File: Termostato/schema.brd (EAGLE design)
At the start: 100 x 80 mm, 11 parts, among them K1 RELAY-SPDT-JZC-11F

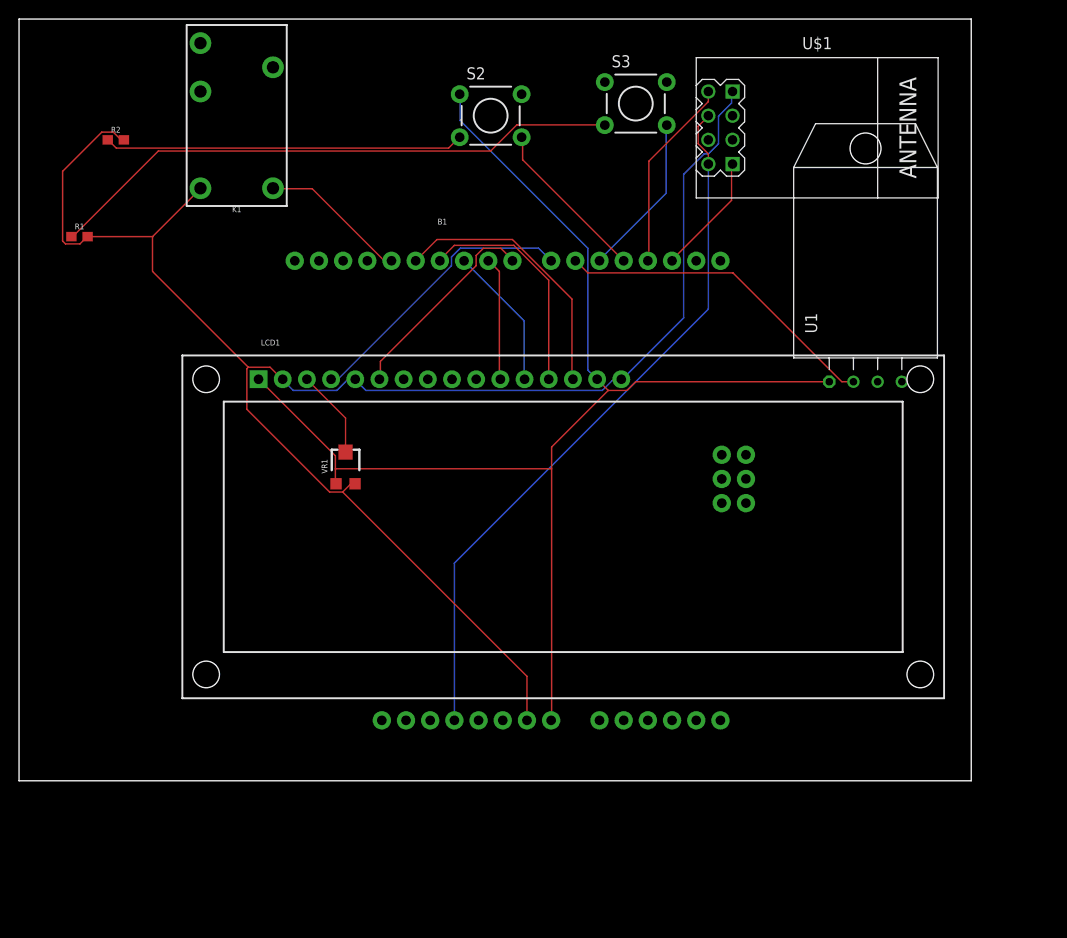
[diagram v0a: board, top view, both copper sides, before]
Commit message: Arduino shield
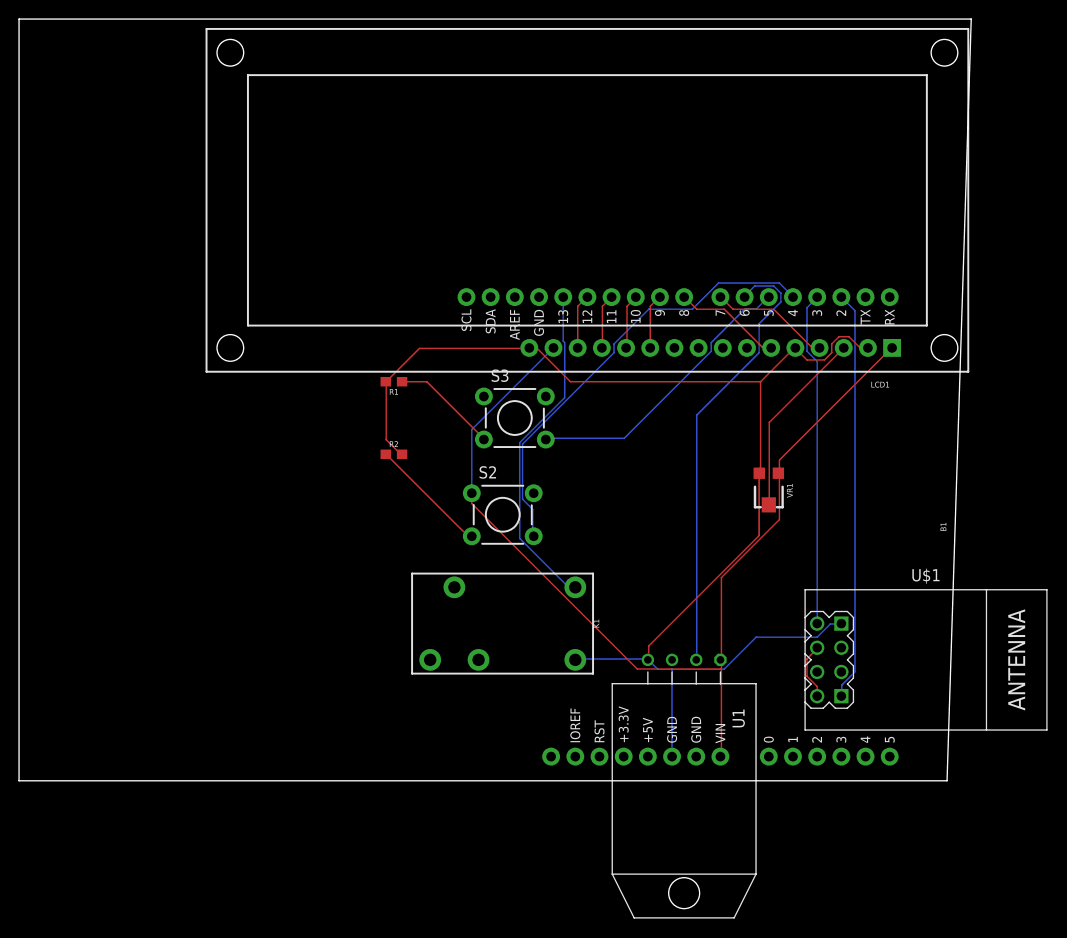
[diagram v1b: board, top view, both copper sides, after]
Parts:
- B1: value ARDUINO_UNO_R3NO_HOLES -> ARDUINO_UNO_R3_SHIELDBASIC; device SparkFun-Boards:ARDUINO_R3_NO_HOLES -> SparkFun-Boards:UNO_R3_SHIELD
- moved K1 60.8 mm to (49.5, 16.5), turned to 90 degrees
- moved U$1 57.0 mm to (95.2, 12.7)
- moved VR1 44.5 mm to (78.7, 30.5), turned to 180 degrees
- moved R2 44.1 mm to (39.4, 34.3)
- moved S2 41.9 mm to (50.8, 27.9)
- moved R1 36.4 mm to (39.4, 41.9), turned to 180 degrees
- moved S3 35.4 mm to (52.1, 38.1)
- moved U1 34.9 mm to (69.8, 12.7), turned to 180 degrees
- moved LCD1 34.4 mm to (59.7, 61.0), turned to 180 degrees
- moved B1 21.9 mm to (66.0, 26.7), turned to 270 degrees
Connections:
- net 3.3V: no longer B1.3.3V
- net GND: now also B1.GND@0; no longer B1.GND@2
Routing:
- net 3.3V: track 75.4 -> 5.96 mm
- net N$4: track 60.9 -> 11.1 mm
- net GND: track 179.7 -> 139.8 mm
- net VCC: track 135.4 -> 104.0 mm
- net RX: track 12.8 -> 43.1 mm
- net D4: track 17.4 -> 46.7 mm
- net N$2: track 37.8 -> 12.6 mm
- net D12: track 28.4 -> 5.78 mm
- net D13: track 15.6 -> 35.4 mm
- net D11: track 24.1 -> 5.75 mm
- net D7: track 29.9 -> 12.6 mm
- net TX: track 20.4 -> 35.2 mm
- net D5: track 17.2 -> 30.2 mm
- net N$3: track 34.5 -> 46.8 mm
- net D8: track 22.0 -> 11.4 mm
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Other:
- outline, holes or cut-outs redrawn
